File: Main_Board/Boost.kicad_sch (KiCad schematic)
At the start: 13 parts, among them U5 TLV61070ADBV

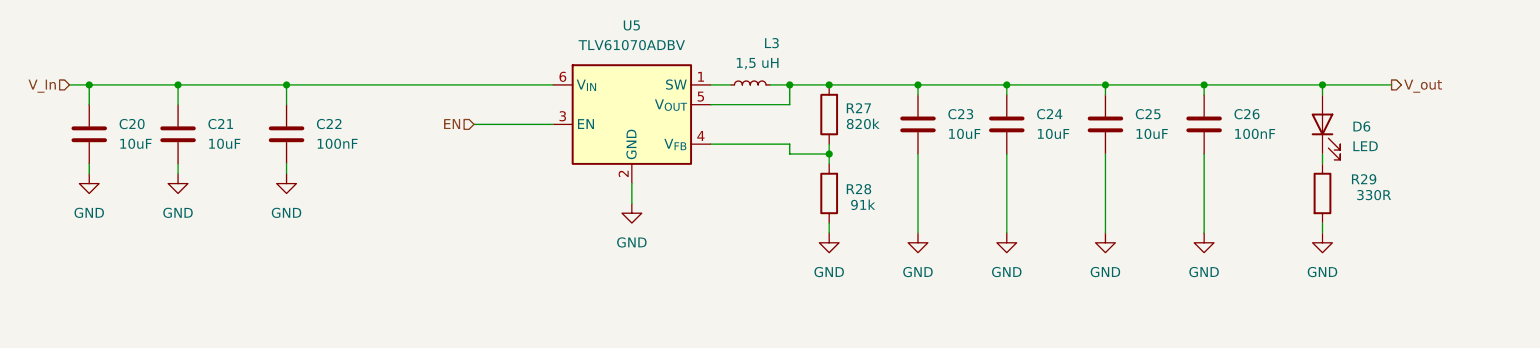
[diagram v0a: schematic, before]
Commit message: Fix schematic readibility
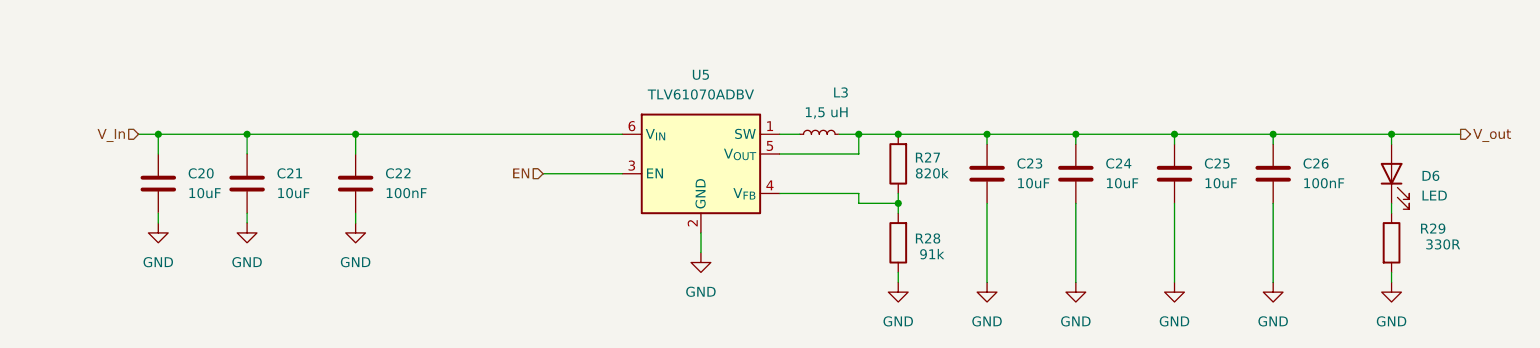
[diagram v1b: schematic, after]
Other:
- moved on the sheet: C20, C21, C22, C23, C24, C25, C26, D6, L3, R27, R28, R29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
